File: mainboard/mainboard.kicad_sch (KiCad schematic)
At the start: 14 parts, among them J1 USB_B_Micro, J2 Conn_Coaxial_Small, SW1 SW_Push, SW2 SW_Push, U1 AMS1117-3.3, U2 STM32MP131AAEx, U3 SX1276, U4 nRF8001, U5 BQ25570, Y1 Crystal_Small

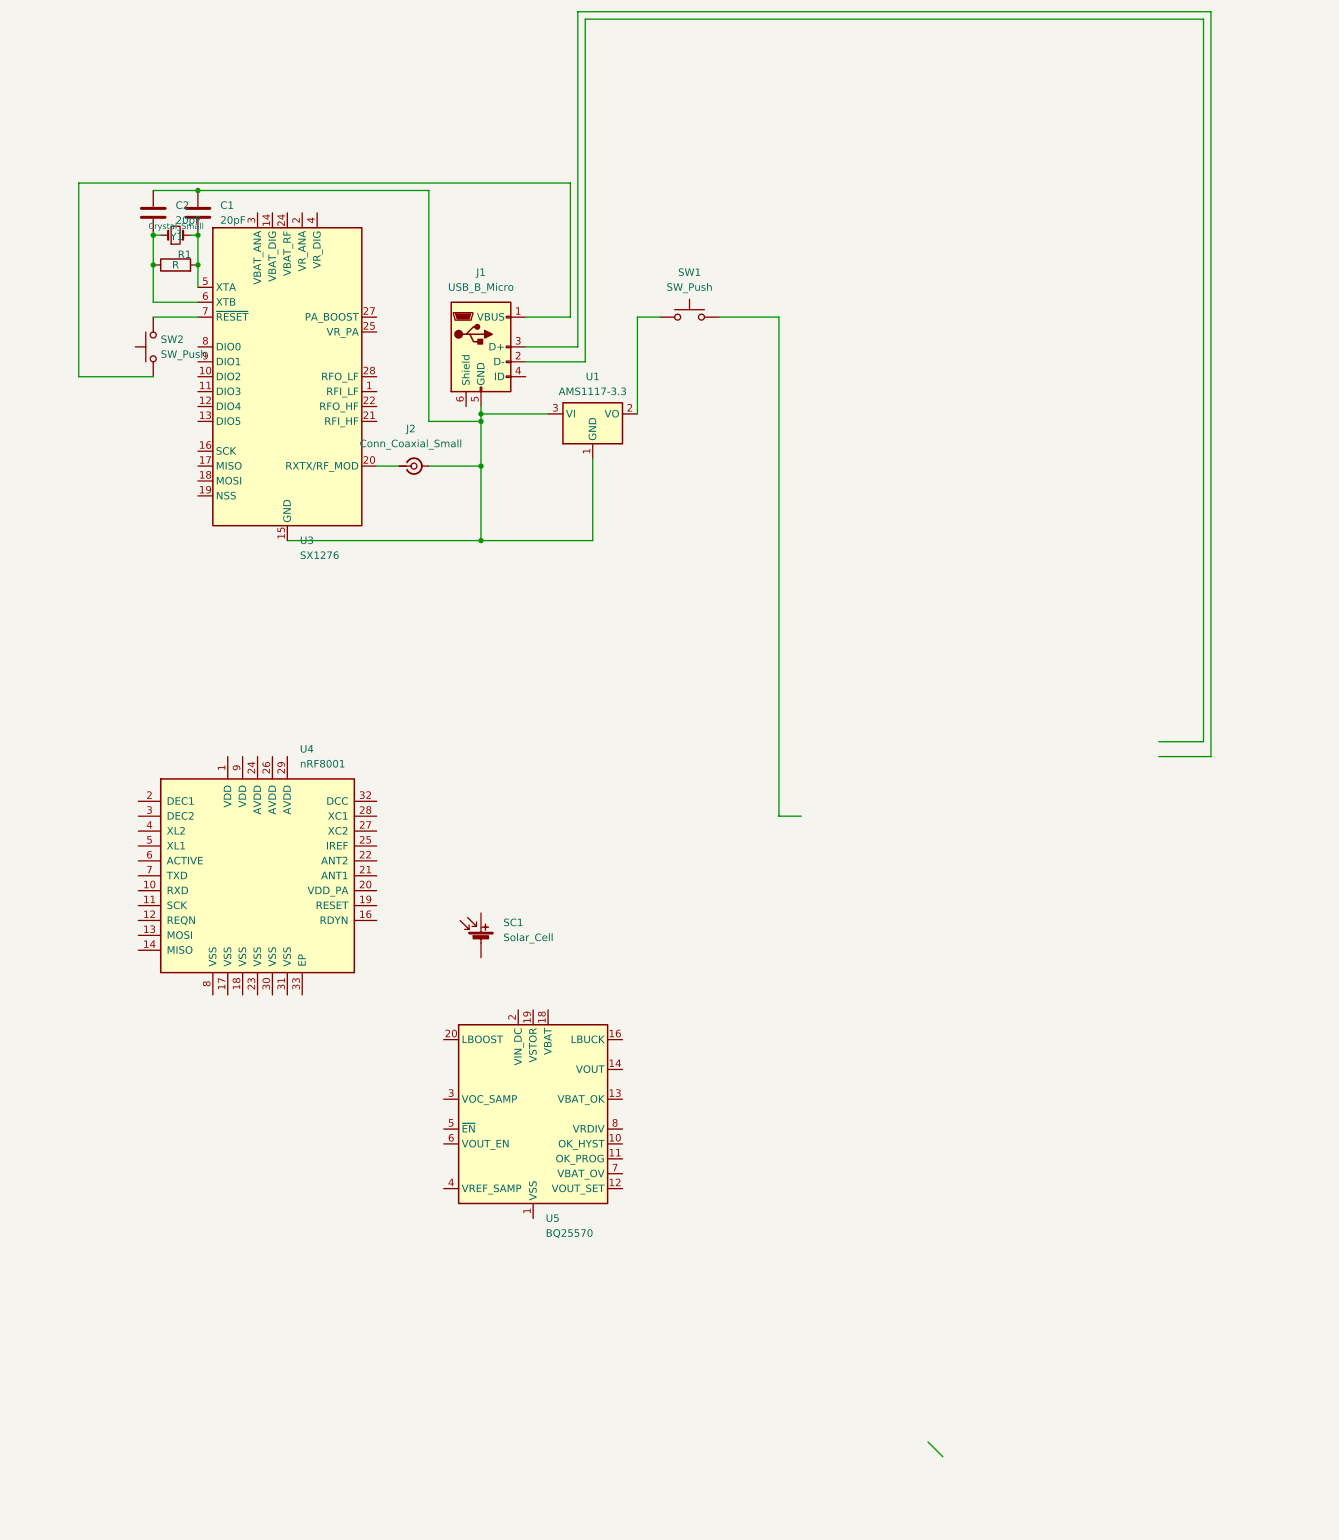
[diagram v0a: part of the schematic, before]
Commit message: Added Proof-Of-Concept
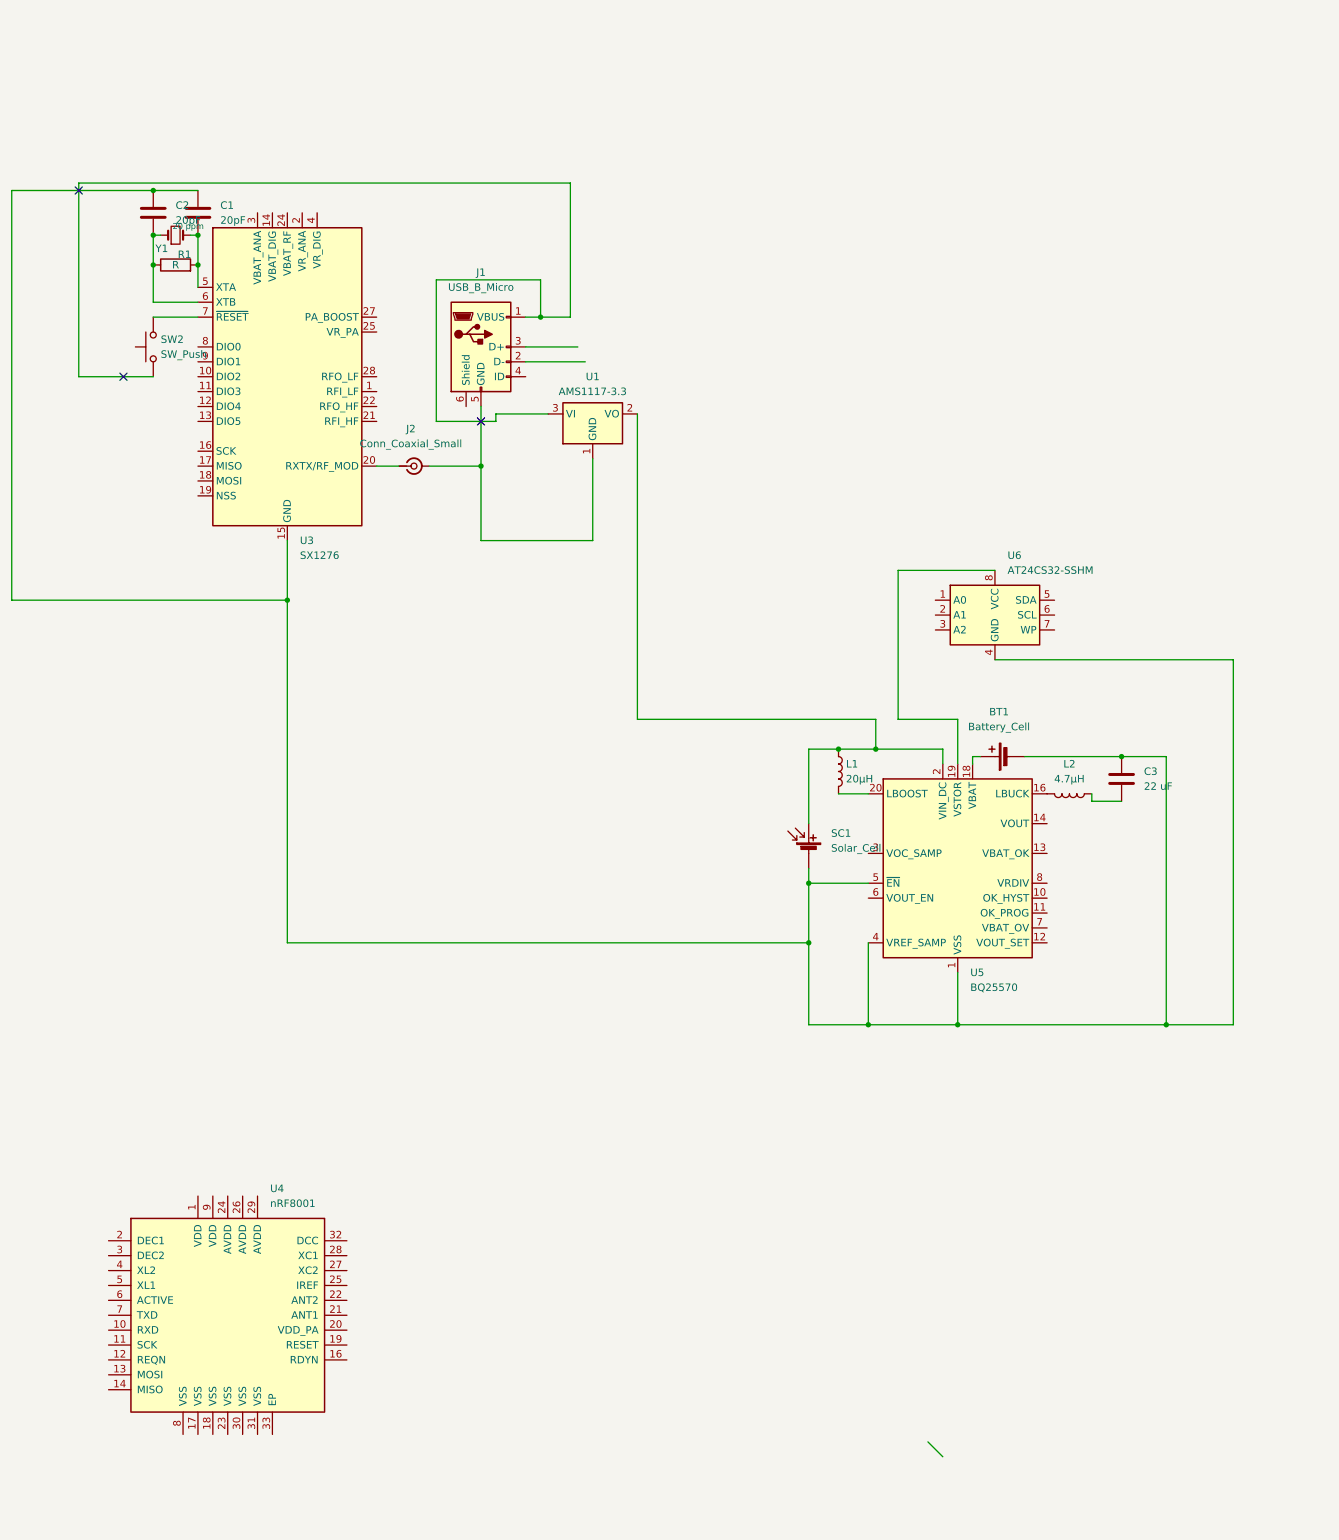
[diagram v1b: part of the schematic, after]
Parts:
- removed SW1: SW_Push, Button_Switch_SMD:SW_SPST_SKQG_WithoutStem, symbol Switch:SW_Push
- added BT1: Battery_Cell, symbol Device:Battery_Cell
- added C3: 22 uF, Capacitor_SMD:C_01005_0402Metric, symbol Device:C
- added L1: 20μH, symbol Device:L
- added L2: 4.7μH, Inductor_SMD_Wurth:L_Wurth_WE-LQSH-2010, symbol Device:L
- added U6: AT24CS32-SSHM, Package_SO:SOIC-8_3.9x4.9mm_P1.27mm, symbol Memory_EEPROM:AT24CS32-SSHM
- Y1: value Crystal_Small -> 20 ppm
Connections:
- net at C1.1, C2.1, U3.15 (GND)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: now also SC1.2 (-), U5.1 (VSS), U5.15 (VSS), U5.17 (VSS), U5.21 (VSS), U5.4 (VREF_SAMP), U5.5 (~{EN}), U5.9 (VSS), BT1.2 (-), C3.1, U6.4 (GND); no longer J1.5 (GND), J2.2 (Ext), U1.1 (GND), U1.3 (VI)
- net at U1.2 (VO): now also SC1.1 (+), U5.2 (VIN_DC), L1.1
- net at J1.1 (VBUS), SW2.1: now also U1.3 (VI)
- net at U5.16 (LBUCK): now also L2.2
- net at U5.18 (VBAT): now also BT1.1 (+)
- net at U5.19 (VSTOR): now also U6.8 (VCC)
- net at U5.20 (LBOOST): now also L1.2
- new net: J1.5 (GND), J2.2 (Ext), U1.1 (GND)
- new net: C3.2, L2.1
- no-connect marks 0 -> 3
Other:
- moved on the sheet: SC1, U4, U5
